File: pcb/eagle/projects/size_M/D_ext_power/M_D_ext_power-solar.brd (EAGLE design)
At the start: 30 parts

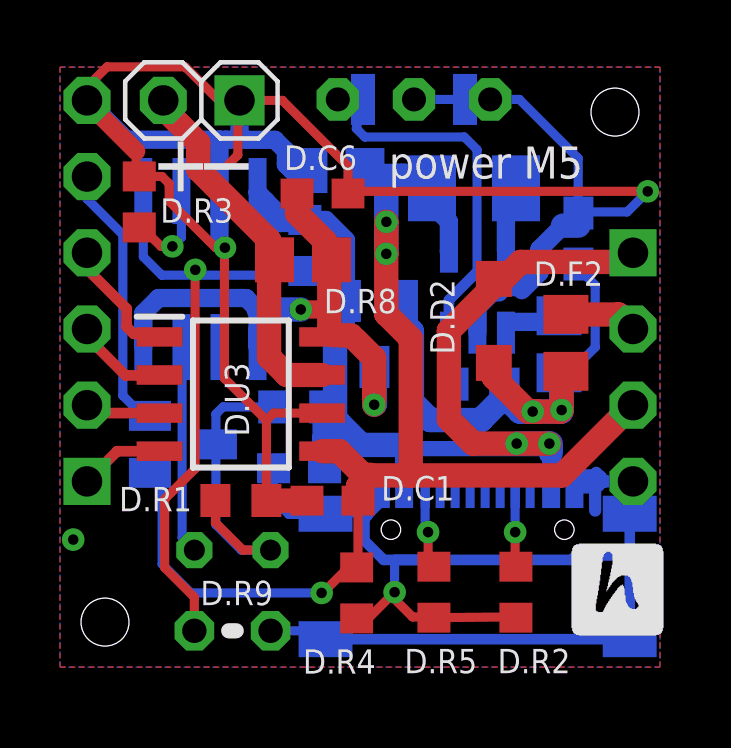
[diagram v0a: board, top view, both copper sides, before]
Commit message: minor changes for PCB v6.
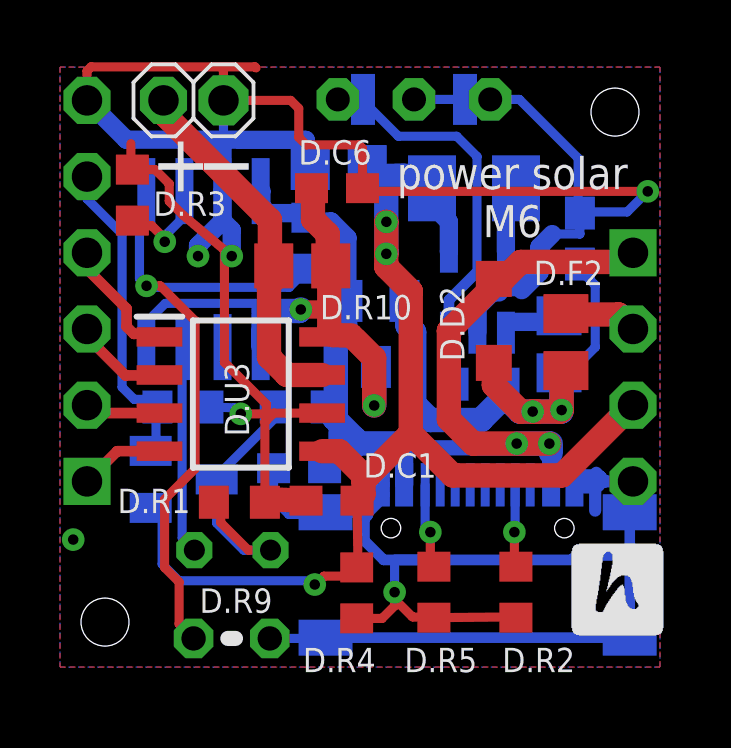
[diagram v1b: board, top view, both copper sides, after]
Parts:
- added D.R11: 100k, rcl:R0603
- D.LIPOL: device pinhead2:1X02 -> pinhead2:1X02-2
- D.R10: value 10k? -> 0.1; device rcl:R0603 -> rcl:R0805
- D.R8: value 0.1 -> 10k?; device rcl:R0805 -> rcl:R0603
- moved D.T2 1.17 mm to (4.62, 6.76)
- moved D.R10 0.69 mm to (8.58, 13.9), flipped to the top, turned to 180 degrees
- moved D.R8 0.58 mm to (8.76, 14.6), flipped to the bottom, turned to 90 degrees
- moved D.C6 0.51 mm to (9.73, 16.5)
- moved D.R3 0.32 mm to (2.91, 16.2)
- moved D.LIPOL 0.26 mm to (4.95, 19.4)
- moved D.R9 0.26 mm to (6.22, 1.46)
- moved D.C7 0.13 mm to (9.79, 17.2)
- moved U$2 0.10 mm to (5.28, 13.8)
- moved D.R1 0.08 mm to (6.48, 5.99)
- moved D.R6 0.05 mm to (8.51, 9.17)
- moved D.T1 0.05 mm to (11.0, 11.6)
- moved U$1 0.05 mm to (14.4, 2.75)
- moved D.C2 0.05 mm to (17.8, 14.8)
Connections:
- net GND: now also D.R11.2
- net IN+: now also D.R10.2; no longer D.R8.2
- net IN-: now also D.R10.1; no longer D.R8.1
- net N$1: now also D.R11.1
- net N$8: now also D.R8.1; no longer D.R10.1
- net VUSB: now also D.R8.2; no longer D.R10.2
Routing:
- net GND: track 122.8 -> 125.8 mm, vias 4 -> 6
- net VCC: track 45.4 -> 42.4 mm
- net N$1: track 8.98 -> 10.9 mm
- net N$8: track 20.9 -> 22.5 mm
- net PA3: track 10.9 -> 9.78 mm
- net N$5: track 14.7 -> 13.8 mm
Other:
- board text added: "power solar M6"
- board text removed: "power M5"

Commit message: formal changes
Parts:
- D.R1: value 4k7 -> 5k1
- D.R7: value 390k -> 100k
